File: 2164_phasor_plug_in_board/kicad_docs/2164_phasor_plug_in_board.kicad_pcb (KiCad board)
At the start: 2 copper layers, 58.4 x 50.8 mm, 85 parts, among them J1 Conn_01x04_Male, J2 Conn_01x04_Male, J3 Conn_01x04_Male, J4 Conn_01x08_Male, U1 TL074, U2 SSM2164, U3 TL074, U4 SSM2164, U5 TL074, U6 TL072

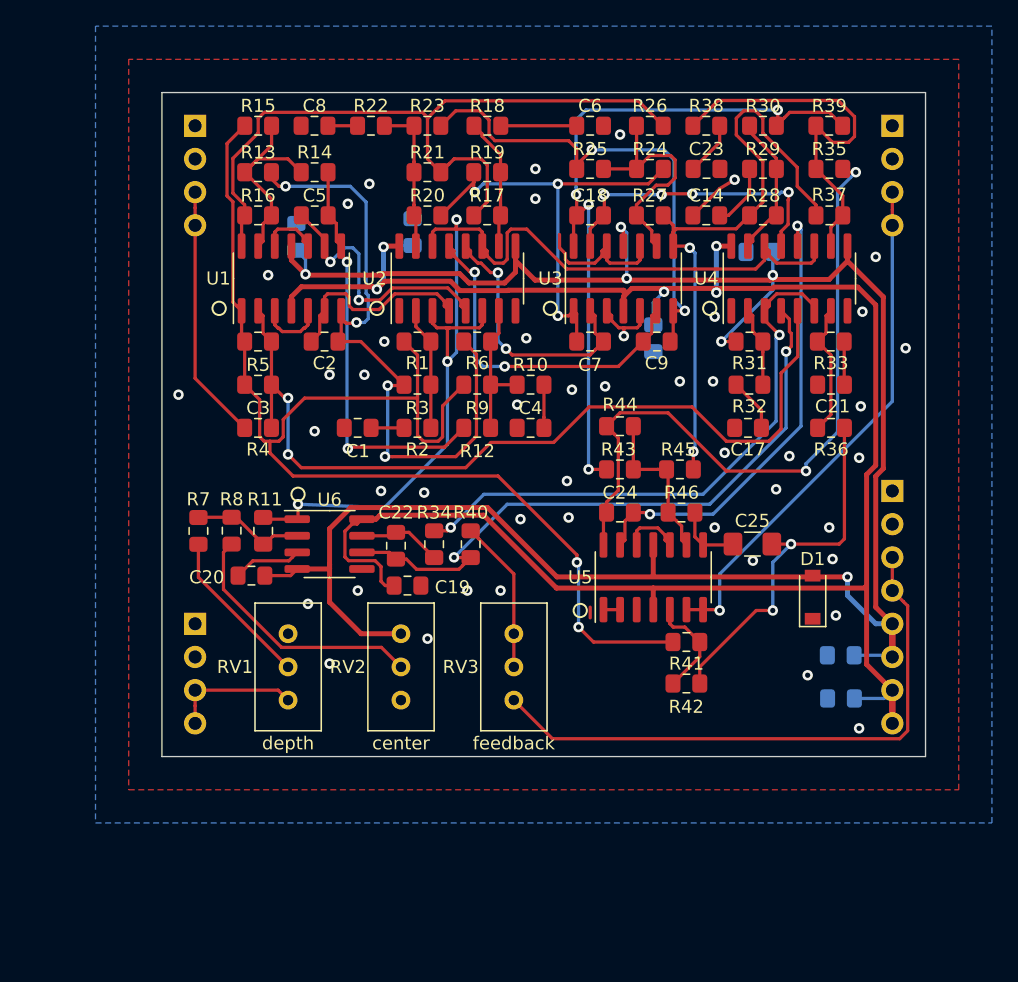
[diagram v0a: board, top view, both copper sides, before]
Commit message: update 2164 phasor board
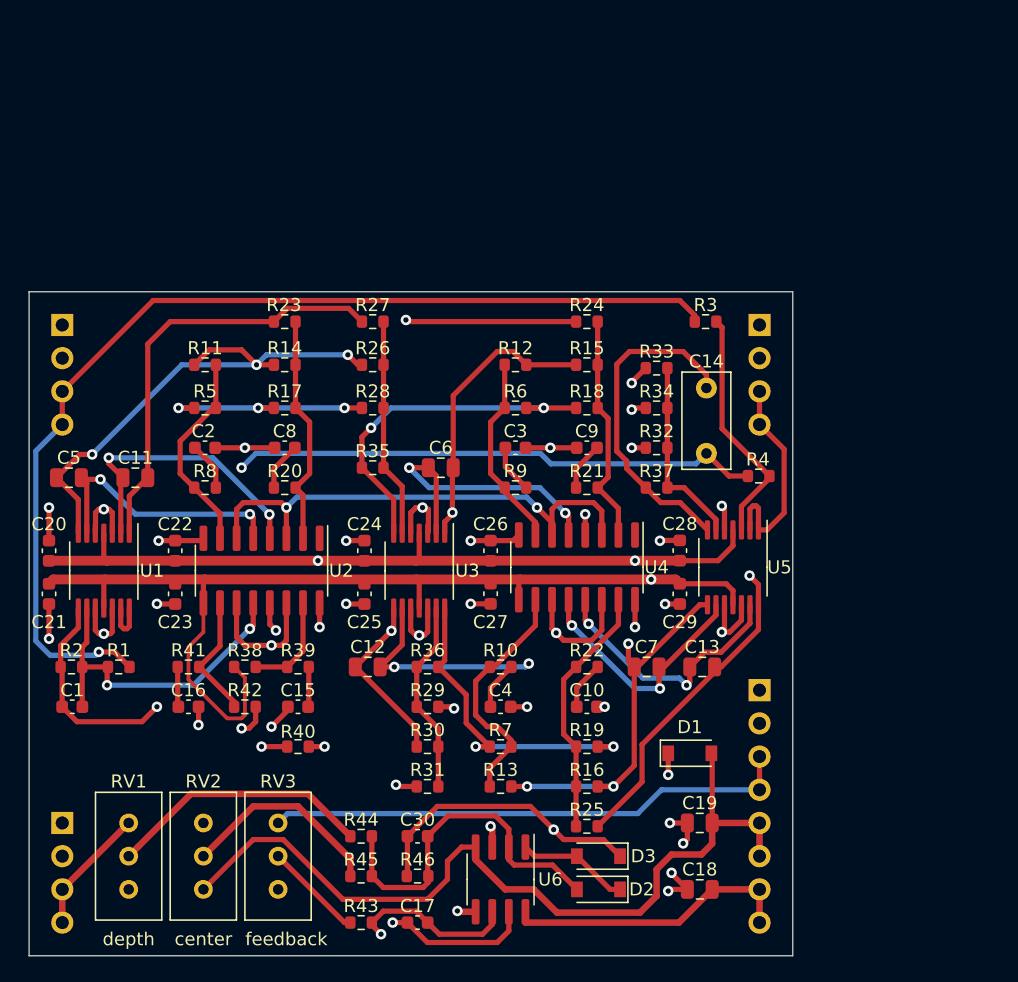
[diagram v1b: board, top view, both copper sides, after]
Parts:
- added C26: 100n, Capacitor_SMD:C_0603_1608Metric, F.Cu at (126.7, 85.9)
- added C27: 100n, Capacitor_SMD:C_0603_1608Metric, F.Cu at (126.7, 89.1)
- added C28: 100n, Capacitor_SMD:C_0603_1608Metric, F.Cu at (141.2, 85.8)
- added C29: 100n, Capacitor_SMD:C_0603_1608Metric, F.Cu at (141.2, 89.2)
- added C30: 100p, Capacitor_SMD:C_0603_1608Metric, F.Cu at (121.2, 107.7)
- added D2: 1N4148W, Diode_SMD:D_SOD-123, F.Cu at (135.0, 111.8)
- added D3: 1N4148W, Diode_SMD:D_SOD-123, F.Cu at (135.0, 109.2)
- C1: value 560pF -> 470p; footprint Capacitor_SMD:C_0805_2012Metric_Pad1.15x1.40mm_HandSolder -> Capacitor_SMD:C_0603_1608Metric
- C10, C15, C16: value 100nF -> 1n2; footprint Capacitor_SMD:C_0805_2012Metric_Pad1.15x1.40mm_HandSolder -> Capacitor_SMD:C_0603_1608Metric; moved to F.Cu
- C11, C12, C13: value 100nF -> 220p; footprint Capacitor_SMD:C_0805_2012Metric_Pad1.15x1.40mm_HandSolder -> Capacitor_SMD:C_0805_2012Metric; moved to F.Cu
- C14: value 560pF -> 470n; footprint Capacitor_SMD:C_0805_2012Metric_Pad1.15x1.40mm_HandSolder -> Capacitor_THT:C_Rect_L7.2mm_W3.5mm_P5.00mm_FKS2_FKP2_MKS2_MKP2
- C17, C4, C8: value 560pF -> 1n2; footprint Capacitor_SMD:C_0805_2012Metric_Pad1.15x1.40mm_HandSolder -> Capacitor_SMD:C_0603_1608Metric
- C18: value 220pF -> 10u; footprint Capacitor_SMD:C_0805_2012Metric_Pad1.15x1.40mm_HandSolder -> Capacitor_SMD:C_0805_2012Metric
- C19: value 100nF -> 10u; footprint Capacitor_SMD:C_0805_2012Metric_Pad1.15x1.40mm_HandSolder -> Capacitor_SMD:C_0805_2012Metric
- C2, C9: value 220pF -> 1n2; footprint Capacitor_SMD:C_0805_2012Metric_Pad1.15x1.40mm_HandSolder -> Capacitor_SMD:C_0603_1608Metric
- C20: value 100nF -> 100n; footprint Capacitor_SMD:C_0805_2012Metric_Pad1.15x1.40mm_HandSolder -> Capacitor_SMD:C_0603_1608Metric
- C21, C23: value 560pF -> 100n; footprint Capacitor_SMD:C_0805_2012Metric_Pad1.15x1.40mm_HandSolder -> Capacitor_SMD:C_0603_1608Metric
- C22: value 100pF -> 100n; footprint Capacitor_SMD:C_0805_2012Metric_Pad1.15x1.40mm_HandSolder -> Capacitor_SMD:C_0603_1608Metric
- C24: value 220pF -> 100n; footprint Capacitor_SMD:C_0805_2012Metric_Pad1.15x1.40mm_HandSolder -> Capacitor_SMD:C_0603_1608Metric
- C25: value 220nF -> 100n; footprint Capacitor_SMD:C_1206_3216Metric_Pad1.42x1.75mm_HandSolder -> Capacitor_SMD:C_0603_1608Metric
- C3: value 470pF -> 1n2; footprint Capacitor_SMD:C_0805_2012Metric_Pad1.15x1.40mm_HandSolder -> Capacitor_SMD:C_0603_1608Metric
- C5, C7: value 220pF -> 220p; footprint Capacitor_SMD:C_0805_2012Metric_Pad1.15x1.40mm_HandSolder -> Capacitor_SMD:C_0805_2012Metric
- C6: value 560pF -> 220p; footprint Capacitor_SMD:C_0805_2012Metric_Pad1.15x1.40mm_HandSolder -> Capacitor_SMD:C_0805_2012Metric
- J1: value Conn_01x04_Male -> signal_in
- J2: value Conn_01x04_Male -> CV_in
- J3: value Conn_01x04_Male -> signal_out
- J4: value Conn_01x08_Male -> feedback_CV_and_PS
- R1, R12, R17, R19, R23, R3, R5: footprint Resistor_SMD:R_0805_2012Metric_Pad1.15x1.40mm_HandSolder -> Resistor_SMD:R_0603_1608Metric
- R10, R22: value 510 -> 220; footprint Resistor_SMD:R_0805_2012Metric_Pad1.15x1.40mm_HandSolder -> Resistor_SMD:R_0603_1608Metric
- R11, R7: value 100k -> 30k; footprint Resistor_SMD:R_0805_2012Metric_Pad1.15x1.40mm_HandSolder -> Resistor_SMD:R_0603_1608Metric
- R13, R24, R25: value 10k -> 30k; footprint Resistor_SMD:R_0805_2012Metric_Pad1.15x1.40mm_HandSolder -> Resistor_SMD:R_0603_1608Metric
- R14: value 10k -> 15k; footprint Resistor_SMD:R_0805_2012Metric_Pad1.15x1.40mm_HandSolder -> Resistor_SMD:R_0603_1608Metric
- R15, R16: value 20k -> 15k; footprint Resistor_SMD:R_0805_2012Metric_Pad1.15x1.40mm_HandSolder -> Resistor_SMD:R_0603_1608Metric
- R18, R2: value 510 -> 30k; footprint Resistor_SMD:R_0805_2012Metric_Pad1.15x1.40mm_HandSolder -> Resistor_SMD:R_0603_1608Metric
- R20: value 15k -> 220; footprint Resistor_SMD:R_0805_2012Metric_Pad1.15x1.40mm_HandSolder -> Resistor_SMD:R_0603_1608Metric
- R21, R39, R41, R9: value 30k -> 220; footprint Resistor_SMD:R_0805_2012Metric_Pad1.15x1.40mm_HandSolder -> Resistor_SMD:R_0603_1608Metric
- R26, R27: value 20k -> 10k; footprint Resistor_SMD:R_0805_2012Metric_Pad1.15x1.40mm_HandSolder -> Resistor_SMD:R_0603_1608Metric
- R28, R36, R37: value 30k -> 20k; footprint Resistor_SMD:R_0805_2012Metric_Pad1.15x1.40mm_HandSolder -> Resistor_SMD:R_0603_1608Metric
- R29, R32, R33: value 510 -> 10k; footprint Resistor_SMD:R_0805_2012Metric_Pad1.15x1.40mm_HandSolder -> Resistor_SMD:R_0603_1608Metric
- R30: value 30k -> 10k; footprint Resistor_SMD:R_0805_2012Metric_Pad1.15x1.40mm_HandSolder -> Resistor_SMD:R_0603_1608Metric
- R31: value 270k -> 20k; footprint Resistor_SMD:R_0805_2012Metric_Pad1.15x1.40mm_HandSolder -> Resistor_SMD:R_0603_1608Metric
- R34: value 4k7 -> 20k; footprint Resistor_SMD:R_0805_2012Metric_Pad1.15x1.40mm_HandSolder -> Resistor_SMD:R_0603_1608Metric
- R35: value 15k -> 20k; footprint Resistor_SMD:R_0805_2012Metric_Pad1.15x1.40mm_HandSolder -> Resistor_SMD:R_0603_1608Metric
- R38: value 510 -> 270k; footprint Resistor_SMD:R_0805_2012Metric_Pad1.15x1.40mm_HandSolder -> Resistor_SMD:R_0603_1608Metric
- R4: value 30k -> 12k; footprint Resistor_SMD:R_0805_2012Metric_Pad1.15x1.40mm_HandSolder -> Resistor_SMD:R_0603_1608Metric
- R40: value 51k -> 4k7; footprint Resistor_SMD:R_0805_2012Metric_Pad1.15x1.40mm_HandSolder -> Resistor_SMD:R_0603_1608Metric
- R42: value 12k -> 30k; footprint Resistor_SMD:R_0805_2012Metric_Pad1.15x1.40mm_HandSolder -> Resistor_SMD:R_0603_1608Metric
- R43: value 10k -> 51k; footprint Resistor_SMD:R_0805_2012Metric_Pad1.15x1.40mm_HandSolder -> Resistor_SMD:R_0603_1608Metric
- R44: value 10k -> 100k; footprint Resistor_SMD:R_0805_2012Metric_Pad1.15x1.40mm_HandSolder -> Resistor_SMD:R_0603_1608Metric
- R45: value 20k -> 680k; footprint Resistor_SMD:R_0805_2012Metric_Pad1.15x1.40mm_HandSolder -> Resistor_SMD:R_0603_1608Metric
- R46: value 20k -> 150k; footprint Resistor_SMD:R_0805_2012Metric_Pad1.15x1.40mm_HandSolder -> Resistor_SMD:R_0603_1608Metric
- R6: value 15k -> 30k; footprint Resistor_SMD:R_0805_2012Metric_Pad1.15x1.40mm_HandSolder -> Resistor_SMD:R_0603_1608Metric
- R8: value 330k -> 220; footprint Resistor_SMD:R_0805_2012Metric_Pad1.15x1.40mm_HandSolder -> Resistor_SMD:R_0603_1608Metric
- RV2, RV3: value 100k -> 10k
- U1, U3, U5: footprint Package_SO:SOIC-14_3.9x8.7mm_P1.27mm -> Package_SO:TSSOP-14_4.4x5mm_P0.65mm
- U2, U4: value SSM2164 -> SSI2164
- moved C21 61.9 mm to (93.0, 89.2), turned to 90 degrees
- moved R39 55.7 mm to (112.0, 94.7), turned to 0 degrees
- moved C11 55.7 mm to (99.6, 80.3), turned to 180 degrees
- moved R38 54.4 mm to (108.0, 94.7)
- moved J2 54.3 mm to (94.0, 106.7)
- moved R30 54.0 mm to (121.9, 100.8)
- moved C18 52.2 mm to (142.7, 111.8), turned to 180 degrees
- moved C23 52.1 mm to (102.6, 89.2), turned to 90 degrees
- moved R13 50.5 mm to (127.5, 103.9), turned to 180 degrees
- moved R16 50.4 mm to (134.1, 103.9)
- moved R25 50.3 mm to (134.1, 106.9)
- moved R29 48.5 mm to (121.9, 97.8), turned to 0 degrees
- moved C17 45.5 mm to (121.2, 114.3), turned to 0 degrees
- moved R19 44.6 mm to (134.1, 100.8)
- moved R22 44.6 mm to (134.1, 94.7), turned to 0 degrees
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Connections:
- net Net-(J4-Pad3) renamed /feedback_VCA/feedback_CV_in
- C1 pad 1: Net-(C1-Pad1) -> /all_pass_stages/signal_v_in
- C1 pad 2: GND -> /feedback_signal
- C10 pad 1: +12V -> Net-(C10-Pad1)
- C11 pad 1: GND -> Net-(C11-Pad1)
- C11 pad 2: -12V -> Net-(C11-Pad2)
- C12 pad 1: +12V -> Net-(C12-Pad1)
- C12 pad 2: GND -> Net-(C12-Pad2)
- C13 pad 1: GND -> Net-(C13-Pad1)
- C13 pad 2: -12V -> Net-(C13-Pad2)
- C14 pad 1: Net-(C14-Pad1) -> /feedback_VCA/feedback_signal_v_in
- C14 pad 2: GND -> Net-(C14-Pad2)
- C15 pad 1: +12V -> Net-(C15-Pad1)
- C16 pad 1: GND -> Net-(C16-Pad1)
- C16 pad 2: -12V -> GND
- C17 pad 2: GND -> Net-(C17-Pad2)
- C18 pad 1: Net-(C18-Pad1) -> +12V
- C18 pad 2: Net-(C18-Pad2) -> GND
- C19 pad 1: +12V -> GND
- C19 pad 2: GND -> -12V
- C2 pad 2: Net-(C2-Pad2) -> GND
- C20 pad 1: GND -> +12V
- C20 pad 2: -12V -> GND
- C21 pad 1: Net-(C21-Pad1) -> GND
- C21 pad 2: GND -> -12V
- C22 pad 1: Net-(C22-Pad1) -> +12V
- C22 pad 2: Net-(C22-Pad2) -> GND
- C23 pad 1: Net-(C23-Pad1) -> GND
- C23 pad 2: GND -> -12V
- C24 pad 1: Net-(C24-Pad1) -> +12V
- C24 pad 2: Net-(C24-Pad2) -> GND
- C25 pad 1: Net-(C25-Pad1) -> GND
- C25 pad 2: Net-(C25-Pad2) -> -12V
- C3 pad 2: Net-(C3-Pad2) -> GND
- C6 pad 2: GND -> Net-(C6-Pad2)
- C9 pad 2: Net-(C9-Pad2) -> GND
- J2 pad 3: Net-(J2-Pad3) -> /CV_scaler/raw_CV_in
- J2 pad 4: Net-(J2-Pad3) -> /CV_scaler/raw_CV_in
- R1 pad 1: Net-(R1-Pad1) -> /feedback_signal
- R1 pad 2: Net-(C3-Pad1) -> Net-(J1-Pad3)
- R11 pad 1: Fcv -> Net-(C5-Pad1)
- R12 pad 1: Net-(C5-Pad1) -> Net-(C6-Pad1)
- R12 pad 2: Net-(R10-Pad1) -> Net-(R12-Pad2)
- R13 pad 1: Net-(R13-Pad1) -> Net-(C7-Pad1)
- R13 pad 2: Net-(C2-Pad1) -> Net-(R10-Pad1)
- R14 pad 1: Net-(R13-Pad1) -> Net-(R14-Pad1)
- R15 pad 1: Net-(R13-Pad1) -> Net-(R15-Pad1)
- R15 pad 2: Net-(C3-Pad1) -> Net-(C6-Pad1)
- R16 pad 2: Net-(R13-Pad1) -> Net-(C7-Pad1)
- R17 pad 1: Net-(R17-Pad1) -> Net-(R14-Pad1)
- R17 pad 2: Net-(R16-Pad1) -> /all_pass_stages/signal_v_in
- R18 pad 1: Net-(R17-Pad1) -> Net-(R15-Pad1)
- R18 pad 2: Net-(C6-Pad1) -> Net-(R18-Pad2)
- R19 pad 1: Net-(C7-Pad1) -> Net-(R16-Pad1)
- R19 pad 2: Net-(R17-Pad1) -> Net-(R19-Pad2)
- R2 pad 1: Net-(R1-Pad1) -> /all_pass_stages/signal_v_in
- R2 pad 2: Net-(C1-Pad1) -> /feedback_signal
- R20 pad 1: Net-(R20-Pad1) -> Net-(R14-Pad1)
- R20 pad 2: Net-(C7-Pad1) -> Net-(C8-Pad1)
- R21 pad 1: Net-(R20-Pad1) -> Net-(R15-Pad1)
- R21 pad 2: Net-(R16-Pad1) -> Net-(C9-Pad1)
- R22 pad 1: Net-(R20-Pad1) -> Net-(R16-Pad1)
- R22 pad 2: Net-(C8-Pad1) -> Net-(C10-Pad1)
- R23 pad 1: Net-(C9-Pad1) -> Net-(C11-Pad1)
- R23 pad 2: Net-(R20-Pad1) -> Net-(R14-Pad1)
- R24 pad 1: Net-(R24-Pad1) -> Net-(C12-Pad1)
- R24 pad 2: Net-(C7-Pad1) -> Net-(R15-Pad1)
- R25 pad 1: Net-(R24-Pad1) -> Net-(C13-Pad1)
- R25 pad 2: Net-(C9-Pad1) -> Net-(R16-Pad1)
- R26 pad 1: Net-(R24-Pad1) -> Net-(R26-Pad1)
- R26 pad 2: Net-(R16-Pad1) -> Net-(C5-Pad1)
- R27 pad 1: Net-(R27-Pad1) -> Net-(R26-Pad1)
- R27 pad 2: Net-(R24-Pad1) -> Net-(C11-Pad1)
- R28 pad 1: Net-(R28-Pad1) -> Net-(R26-Pad1)
- R28 pad 2: Net-(R27-Pad1) -> /all_pass_stages/signal_v_in
- R29 pad 1: Net-(R28-Pad1) -> Net-(R29-Pad1)
- R29 pad 2: Net-(C14-Pad1) -> Net-(C6-Pad1)
- R3 pad 1: Net-(C2-Pad1) -> Net-(J1-Pad3)
- R3 pad 2: Net-(R1-Pad1) -> Net-(R3-Pad2)
- R30 pad 1: Net-(C18-Pad1) -> Net-(R29-Pad1)
- R30 pad 2: Net-(R28-Pad1) -> Net-(C12-Pad1)
- R31 pad 1: -12V -> Net-(R29-Pad1)
- R31 pad 2: Net-(R31-Pad2) -> Net-(R18-Pad2)
- R32 pad 1: Net-(R31-Pad2) -> Net-(R32-Pad1)
- R32 pad 2: Net-(C17-Pad1) -> Net-(C7-Pad1)
- R33 pad 1: Net-(R33-Pad1) -> Net-(R32-Pad1)
- R33 pad 2: Net-(C21-Pad1) -> Net-(C13-Pad1)
- R34 pad 1: Net-(R34-Pad1) -> Net-(R32-Pad1)
- R34 pad 2: Net-(C22-Pad1) -> Net-(R19-Pad2)
- R35 pad 1: Net-(R35-Pad1) -> Net-(R18-Pad2)
- R35 pad 2: Net-(C18-Pad1) -> Net-(R26-Pad1)
- R36 pad 1: Net-(R33-Pad1) -> Net-(R19-Pad2)
- R36 pad 2: Net-(C25-Pad1) -> Net-(R29-Pad1)
- R37 pad 1: Net-(R35-Pad1) -> Net-(C14-Pad2)
- R37 pad 2: Net-(R27-Pad1) -> Net-(R32-Pad1)
- R38 pad 1: Net-(R35-Pad1) -> -12V
- R38 pad 2: Net-(C23-Pad1) -> Net-(R38-Pad2)
- R39 pad 1: Net-(C24-Pad1) -> Net-(R38-Pad2)
- R39 pad 2: Net-(R35-Pad1) -> Net-(C15-Pad1)
- R4 pad 1: Net-(C3-Pad2) -> Net-(R3-Pad2)
- R4 pad 2: Net-(J2-Pad3) -> /feedback_VCA/feedback_signal_v_in
- R40 pad 1: Net-(C22-Pad2) -> Net-(R40-Pad1)
- R40 pad 2: Net-(R40-Pad2) -> Net-(C17-Pad1)
- R41 pad 1: Net-(C3-Pad1) -> Net-(R41-Pad1)
- R41 pad 2: Net-(R41-Pad2) -> Net-(C16-Pad1)
- R42 pad 1: Net-(R41-Pad2) -> Net-(R41-Pad1)
- R42 pad 2: Net-(C25-Pad1) -> /feedback_VCA/feedback_signal_v_in
- R43 pad 1: Net-(R43-Pad1) -> Net-(C17-Pad2)
- R43 pad 2: Net-(C18-Pad1) -> Net-(R43-Pad2)
- R44 pad 1: Net-(R43-Pad1) -> Net-(C30-Pad2)
- R44 pad 2: Net-(C24-Pad1) -> Net-(R44-Pad2)
- R45 pad 1: Net-(R43-Pad1) -> Net-(C30-Pad2)
- R45 pad 2: Net-(R27-Pad1) -> Net-(R45-Pad2)
- R46 pad 1: Net-(C25-Pad2) -> /all_pass_stages/Vfc_in
- R46 pad 2: Net-(R43-Pad1) -> Net-(C30-Pad2)
- R5 pad 1: Net-(C3-Pad1) -> Net-(R11-Pad2)
- R5 pad 2: Net-(C3-Pad2) -> /all_pass_stages/signal_v_in
- R6 pad 1: Net-(R10-Pad1) -> Net-(R12-Pad2)
- R6 pad 2: Net-(C2-Pad1) -> Net-(R18-Pad2)
- R7 pad 1: Net-(R11-Pad2) -> Net-(R10-Pad1)
- R7 pad 2: Net-(R7-Pad2) -> Net-(R19-Pad2)
- R8 pad 2: Net-(R8-Pad2) -> Net-(C2-Pad1)
- R9 pad 1: Net-(R10-Pad1) -> Net-(R12-Pad2)
- RV1 pad 2: Net-(R7-Pad2) -> Net-(R44-Pad2)
- RV1 pad 3: Net-(J1-Pad3) -> /CV_scaler/raw_CV_in
- RV2 pad 2: Net-(R8-Pad2) -> Net-(R45-Pad2)
- RV3 pad 1: Net-(R40-Pad2) -> GND
- RV3 pad 2: Net-(R40-Pad2) -> Net-(R43-Pad2)
- U1 pad 1: Net-(C3-Pad1) -> Net-(C11-Pad1)
- U1 pad 13: Net-(R13-Pad1) -> Net-(U1-Pad13)
- U1 pad 14: Net-(R16-Pad1) -> Net-(U1-Pad13)
- U1 pad 2: Net-(C3-Pad2) -> Net-(C11-Pad2)
- U1 pad 6: Net-(C2-Pad2) -> Net-(C5-Pad2)
- U1 pad 7: Net-(C2-Pad1) -> Net-(C5-Pad1)
- U1 pad 8: Net-(C5-Pad1) -> /all_pass_stages/signal_v_in
- U1 pad 9: Net-(C5-Pad2) -> /feedback_signal
- U2 pad 10: Net-(R17-Pad1) -> Net-(R41-Pad1)
- U2 pad 11: Fcv -> Net-(R40-Pad1)
- U2 pad 12: Net-(C7-Pad2) -> /feedback_signal
- U2 pad 13: Net-(C9-Pad2) -> Net-(C17-Pad2)
- U2 pad 14: Fcv -> Net-(R40-Pad1)
- U2 pad 15: Net-(R20-Pad1) -> Net-(R38-Pad2)
- U2 pad 2: Net-(R1-Pad1) -> Net-(R14-Pad1)
- U2 pad 3: Fcv -> /all_pass_stages/Vfc_in
- U2 pad 4: Net-(C2-Pad2) -> Net-(C11-Pad2)
- U2 pad 6: Fcv -> /all_pass_stages/Vfc_in
- U2 pad 7: Net-(R10-Pad1) -> Net-(R11-Pad2)
- U3 pad 1: Net-(C7-Pad1) -> Net-(C6-Pad1)
- U3 pad 13: Net-(C18-Pad2) -> Net-(R29-Pad1)
- U3 pad 14: Net-(C18-Pad1) -> Net-(R19-Pad2)
- U3 pad 2: Net-(C7-Pad2) -> Net-(C6-Pad2)
- U3 pad 6: Net-(C9-Pad2) -> Net-(R26-Pad1)
- U3 pad 7: Net-(C9-Pad1) -> Net-(R18-Pad2)
- U3 pad 8: Net-(R27-Pad1) -> Net-(C12-Pad1)
- U3 pad 9: Net-(R24-Pad1) -> Net-(C12-Pad2)
- U4 pad 10: Net-(R35-Pad1) -> Net-(R10-Pad1)
- U4 pad 11: Fcv -> /all_pass_stages/Vfc_in
- U4 pad 12: Net-(C24-Pad2) -> Net-(C7-Pad2)
- U4 pad 13: Net-(C18-Pad2) -> Net-(C13-Pad2)
- U4 pad 14: Fcv -> /all_pass_stages/Vfc_in
- U4 pad 15: Net-(R28-Pad1) -> Net-(R16-Pad1)
- U4 pad 2: Net-(R31-Pad2) -> Net-(R15-Pad1)
- U4 pad 3: Net-(R34-Pad1) -> /all_pass_stages/Vfc_in
- U4 pad 4: Net-(C22-Pad2) -> Net-(C12-Pad2)
- U4 pad 5: Net-(C3-Pad2) -> Net-(C6-Pad2)
- U4 pad 6: Net-(R34-Pad1) -> /all_pass_stages/Vfc_in
- U4 pad 7: Net-(R33-Pad1) -> Net-(R12-Pad2)
- U5 pad 1: Net-(U5-Pad1) -> Net-(J3-Pad3)
- U5 pad 13: Net-(C24-Pad2) -> Net-(C13-Pad2)
- U5 pad 14: Net-(C24-Pad1) -> Net-(C13-Pad1)
- U5 pad 2: Net-(U5-Pad1) -> Net-(J3-Pad3)
- U5 pad 3: GND -> Net-(R3-Pad2)
- U5 pad 5: Net-(R41-Pad2) -> GND
- U5 pad 6: Net-(J3-Pad3) -> Net-(R32-Pad1)
- U5 pad 7: Net-(J3-Pad3) -> Net-(C14-Pad2)
- U5 pad 8: Net-(C25-Pad2) -> Net-(C7-Pad1)
- U5 pad 9: Net-(R43-Pad1) -> Net-(C7-Pad2)
- U6 pad 1: Fcv -> Net-(D2-Pad1)
- U6 pad 2: Net-(R11-Pad2) -> Net-(C30-Pad2)
- U6 pad 6: Net-(C22-Pad2) -> Net-(C17-Pad2)
- U6 pad 7: Net-(C22-Pad1) -> Net-(C17-Pad1)
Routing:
- net /all_pass_stages/Vfc_in: track 0.00 -> 95.5 mm, vias 0 -> 4
- net Net-(C3-Pad1): track 95.4 -> 3.71 mm, vias 2 -> 0
- net Fcv: track 83.6 -> 0.00 mm, vias 3 -> 0
- net Net-(J1-Pad3): track 9.97 -> 80.4 mm, vias 0 -> 1
- net Net-(C3-Pad2): track 67.0 -> 0.00 mm, vias 2 -> 0
- net /feedback_VCA/feedback_signal_v_in: track 0.00 -> 63.3 mm, vias 0 -> 2
- net Net-(R18-Pad2): track 0.00 -> 56.7 mm, vias 0 -> 3
- net /all_pass_stages/signal_v_in: track 0.00 -> 56.3 mm, vias 0 -> 4
- net Net-(C18-Pad1): track 55.6 -> 0.00 mm, vias 4 -> 0
- net Net-(C24-Pad1): track 53.0 -> 0.00 mm, vias 2 -> 0
- net Net-(R19-Pad2): track 0.00 -> 52.8 mm, vias 0 -> 3
- net Net-(C12-Pad1): track 0.00 -> 51.1 mm, vias 0 -> 2
- net Net-(C22-Pad2): track 49.5 -> 0.00 mm, vias 2 -> 0
- net Net-(R27-Pad1): track 48.9 -> 0.00 mm, vias 2 -> 0
- net Net-(C2-Pad1): track 51.0 -> 3.71 mm, vias 4 -> 0
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- added copper zone on GND_layer_2, net GND
- removed copper zone on B.Cu, net GND
- removed copper zone on F.Cu, net GND
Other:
- copper layers 2 -> 4
- rule pad_to_mask_clearance: 0 -> 0.051
- board text added: "2164 phase shifter rev 0.1 2021-12-08 github.com/JordanAceto/VCF_plug_in_boards"
- board text removed: "2164_phasor_plug_in_board rev1 2019-06-11"
